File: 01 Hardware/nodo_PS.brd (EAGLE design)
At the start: 73 x 93 mm, 31 parts, among them IC1 ATMEGA3208-XU, SW1 EG1213

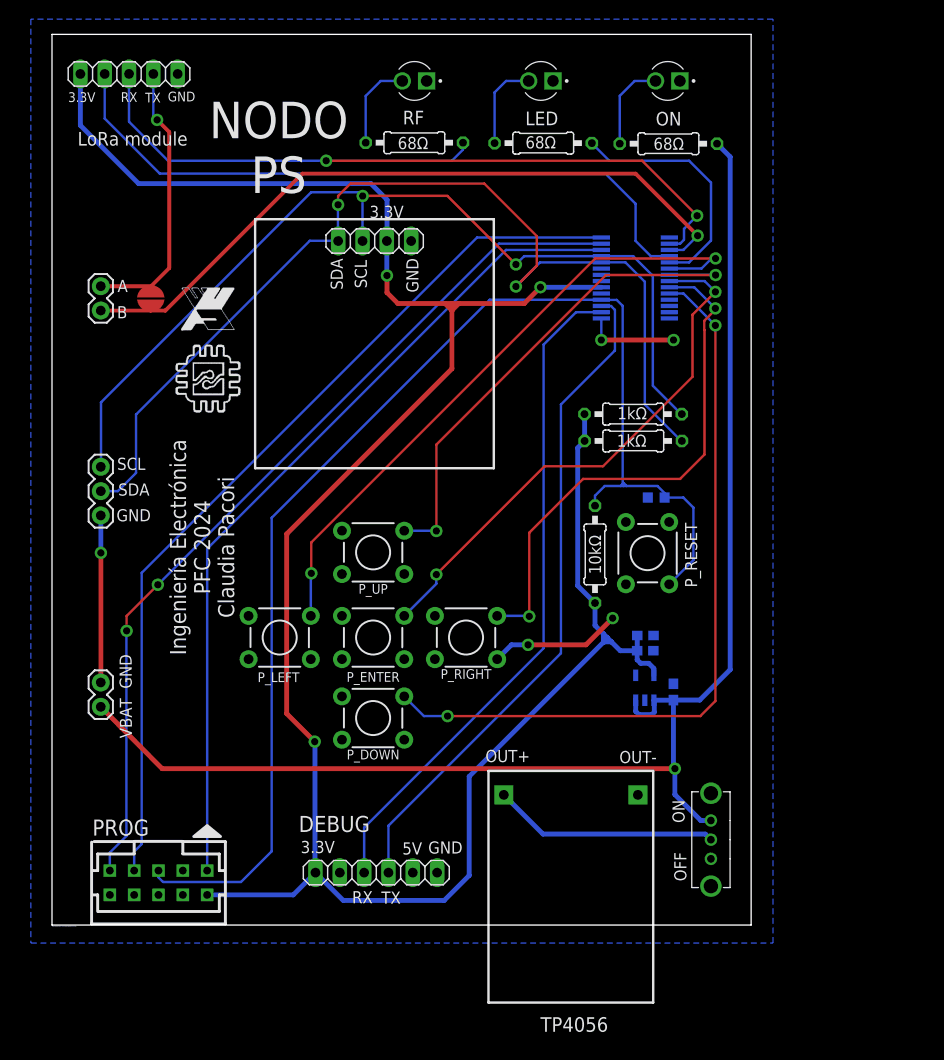
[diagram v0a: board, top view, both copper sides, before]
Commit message: actualizacion de archivos 24-2
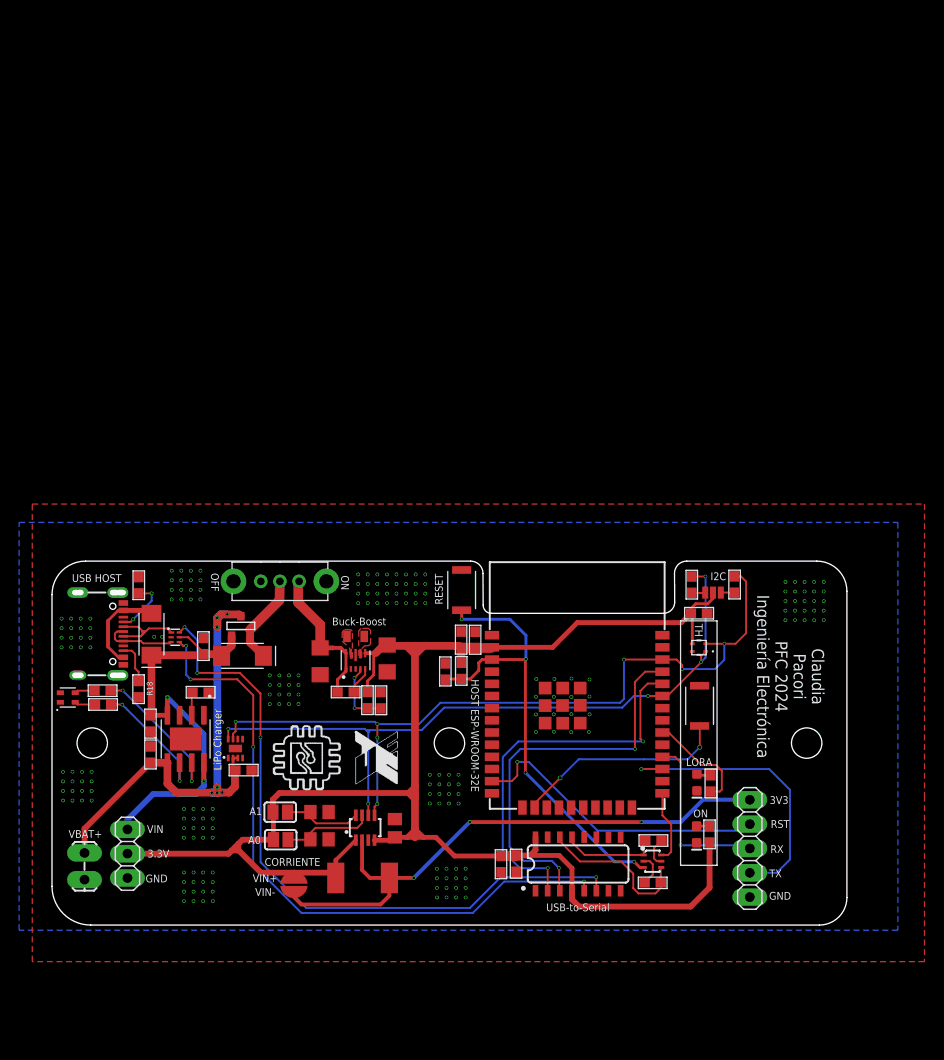
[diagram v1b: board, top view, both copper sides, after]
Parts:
- removed BAT: TP4056MODULE, TP4056MODULE:TP4056MODULE
- removed C4: 1.0uF, SparkFun-Capacitors:0603@3
- removed C5: 0.1uF, SparkFun-Capacitors:0603
- removed DEBUG: (no value), pinhead:1X06
- removed IC1: ATMEGA3208-XU, ATMEGA3208-XU:SOP65P780X200-28N
- removed LORA: REYAX, pinhead:1X05
- removed L_ON1, L_ON2, L_ON3: LED_3MM, LED_3MM:LEDRD254W50D405H1055
- removed OLED: (no value), pinhead:1X04
- removed P_DOWN, P_ENTER, P_LEFT, P_RESET, P_RIGHT, P_UP: MOMENTARY-SWITCH-SPST-PTH-6.0MM, SparkFun-Switches:TACTILE_SWITCH_PTH_6.0MM
- removed R8: 10k, rcl:0207/10
- removed REG: 3.3V, SparkFun-IC-Power:SOT23-5
- removed SV1: (no value), con-harting-ml:3M_10
- removed TP1: (no value), SparkFun-Connectors:1X03
- removed TP3, TP4: (no value), SparkFun-Connectors:1X02
- added A0, A1: (no value), microbuilder:SOLDERJUMPER_REFLOW_NOPASTE
- added C11, C17, C3, C8: 0.1uF, SparkFun-Capacitors:0603
- added C14: 10uF, SparkFun-Capacitors:1206
- added C15: 22uF, SparkFun-Capacitors:1206
- added C16, C18: 4.7uF, SparkFun-Capacitors:0603
- added C2, C7: 10uF, SparkFun-Capacitors:0603
- added D1, D2: BLUE, SparkFun-LED:LED-0603
- added D3, D7: SS34, SparkFun-DiscreteSemi:DO-214AC
- added D5: PRTR5V0U2F, SparkFun-IC-Power:SOT886
- added D8: TJ-S1615SW6TGLCCSRGB-A5, SMD_RGB_:LED_OSTB0603C1C
- added J1: (no value), SparkFun-Connectors:1X02_LOCK_LONGPADS
- added J2: USB Female Type C Connector, SparkFun-Connectors:USB-C-16P_4LAYER-PADS
- added J3: REYAX, pinhead:1X05
- added JP2: (no value), pinhead:1X03
- added L1: 470nH, SparkFun-Coils:0805
- added R10, R12, R22, R23: 220, SparkFun-Resistors:0603
- added R11, R9: 10k, rcl:R0805
- added R13: 511k, SparkFun-Resistors:0603
- added R14: 91k, SparkFun-Resistors:0603
- added R15: 100k, SparkFun-Resistors:0603
- added R18, R19: 5.1k, SparkFun-Resistors:0603
- added R21: 1.2k, SparkFun-Resistors:0603
- added R3, R5: 10k, SparkFun-Resistors:0603
- added S1: EG1213, EG1213:SW_EG1213
- added SENSORCORRIENTE: INA219BIDCNT, microbuilder:SOT23-8
- added SW2: SKRKAEE020, SKRKAEE020:SKRKAEE020
- added T1: AO3401A, zetex:SOT-23
- added TH: SHT40-AD1B-R3, SHT40-AD1B-R3:SHT40AD1BR3
- added TP2: JUMPER-SMT_3_NO_NO-SILK, SparkFun-Jumpers:SMT-JUMPER_3_NO_NO-SILK
- added U11: TPS63802DLAR, TPS63802DLAR:VREG_TPS63802DLAR
- added U13: TP4056, TP4056:SOP127P600X175-9N
- added U2: ESP-WROOM-32E, SparkFun-RF:ESP-WROOM-32D-NARROW
- added U4: CH340C, SparkFun-IC-Comms:SO016
- added U5: MBT3904DW1T1, SparkFun-DiscreteSemi:SC70-6
- added U7: MAX17048, SparkFun-IC-Power:DFN-8
- C1: device rcl:C0603K -> SparkFun-Capacitors:0603
- C6: value 1.0uF -> 0.1uF; device SparkFun-Capacitors:0603@3 -> rcl:C0805
- R1: value 68 -> 0.1/1% (PT2512FK-070R1L); device rcl:0207/10 -> microbuilder:2512
- R2, R4: value 68 -> 10k; device rcl:0207/10 -> SparkFun-Resistors:0603
- R6: value 1k -> 10k; device rcl:0207/10 -> SparkFun-Resistors:0603
- R7: value 1k -> 150k; device rcl:0207/10 -> SparkFun-Resistors:0603
- SW1: value EG1213 -> SKRKAEE020; device EG1213:SW_EG1213 -> SKRKAEE020:SKRKAEE020
- moved R1 83.0 mm to (32.4, 4.92)
- moved JP1 63.0 mm to (25.3, 4.20), turned to 270 degrees
- moved R2 55.8 mm to (42.7, 26.5), turned to 90 degrees
- moved R4 54.5 mm to (66.8, 35.5), turned to 270 degrees
- moved R7 51.0 mm to (15.8, 29.1), turned to 270 degrees
- moved R6 41.8 mm to (62.8, 8.83), turned to 0 degrees
- moved SW1 36.8 mm to (42.8, 35.0), turned to 270 degrees
- moved C6 32.4 mm to (35.8, 10.1), flipped to the top
- moved C1 24.0 mm to (44.2, 29.8), flipped to the top, turned to 90 degrees
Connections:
- removed net DEBUG_RX: DEBUG.3, IC1.16
- removed net DEBUG_TX: DEBUG.4, IC1.17
- removed net LED: IC1.5, R2.1
- removed net LORA_RST: IC1.4, LORA.2
- removed net LORA_RX: IC1.2, LORA.3, R4.1
- removed net LORA_TXA: JP1.2, LORA.4, TP3.1
- removed net LORA_TXB: IC1.3, JP1.1, TP3.2
- removed net MISO: IC1.27, SV1.9
- removed net MOSI: IC1.26, SV1.1
- removed net N$2: L_ON2.A, R1.2
- removed net PULSE_ENTER: IC1.8, P_ENTER.3
- removed net PULSE_LEFT: IC1.6, P_LEFT.3
- removed net PULSE_RIGHT: IC1.9, P_RIGHT.3
- removed net PULS_DOWN: IC1.10, P_DOWN.3
- removed net PULS_UP: IC1.7, P_UP.3
- removed net RESET: C1.1, IC1.18, P_RESET.3, R8.1, SV1.5
- removed net SCK: IC1.28, SV1.7
- removed net SCL: IC1.25, OLED.2, R7.1, TP1.3
- removed net SDA: IC1.24, OLED.1, R6.1, TP1.2
- removed net SS: IC1.1
- removed net V_BATT: C6.1, R1.1, REG.1, REG.3, SW1.3, TP4.2
- new net ADDR0: A0.2, R9.2, SENSORCORRIENTE.7
- new net ADDR1: A1.2, R11.2, SENSORCORRIENTE.8
- new net CC1: J2.B5, R18.2
- new net CC2: J2.A5, R19.2
- new net CH_!CHRG: D8.3, R23.1
- new net CH_!STDBY: D8.2, R22.1
- new net CURRENT_MSR: J3.1, JP1.2, R1.1, SENSORCORRIENTE.2
- new net ESP16_RX2/LORA_TX: J3.4, U2.27
- new net ESP17_TX2/LORA_RX: J3.3, U2.28
- new net ESP1_TX1/USB_RX: U2.35, U4.3
- new net ESP32_!DTR: R6.1, U4.13, U5.1
- new net ESP32_!RTS: R5.1, U4.14, U5.4
- new net ESP32_EN: C3.1, R2.1, SW1.2, U2.3, U5.3
- new net ESP3_RX1/USB_TX: U2.34, U4.2
- new net ESP_0/BOOT: U2.25, U5.6
- new net ESP_13/AUX: SW2.2, U2.16
- new net ESP_14/LORA_RST: J3.2, U2.13
- new net ESP_18/LORA_ST: R12.2, U2.30
- new net ESP_21/SDA: R4.1, SENSORCORRIENTE.6, TH.1, U2.33, U7.8
- new net ESP_22/SCL: R3.1, SENSORCORRIENTE.5, TH.2, U2.36, U7.7
- new net N$10: L1.2, U11.7
- new net N$11: R22.2, U13.6
- new net N$12: R13.1, R14.2, U11.4
- new net N$13: R23.2, U13.7
- new net N$14: R3.2, TP2.3
- new net N$15: R4.2, TP2.1
- new net N$18: R15.1, U11.5
- new net N$24: R6.2, U5.5
- new net N$25: R5.2, U5.2
- new net N$31: R21.2, U13.2
- new net N$4: D5.6, U4.6
- new net N$5: D1.A, R10.1
- new net N$7: D2.A, R12.1
- new net N$8: L1.1, U11.9
- new net USB-C-D+: D5.3, J2.A6, J2.B6
- new net VBAT: C17.1, C18.1, J1.2, T1.1, U13.5, U7.2, U7.3
- new net VBUS: D7.A, J2.VBUS1, J2.VBUS2
- new net VCC: D3.C, S1.2, T1.2
- new net VIN_S: C14.1, R15.2, S1.1, U11.1, U11.10
- net 3.3V: now also A0.1, A1.1, C1.1, C11.1, C15.1, C2.1, C6.1, C7.1, C8.1, JP1.1, JP2.2, R1.2, R10.2, R13.2, R2.2, SENSORCORRIENTE.1, SENSORCORRIENTE.4, TH.3, TP2.2, U11.6, U2.2, U4.16, U4.4; no longer C4.1, C5.2, DEBUG.1, IC1.20, LORA.1, OLED.3, R6.2, R7.2, R8.2, REG.5, SV1.2
- net GND: now also C11.2, C14.2, C15.2, C16.2, C17.2, C18.2, C2.2, C3.2, C7.2, C8.2, D1.C, D2.C, D5.2, D8.4, J1.1, J2.GND, J2.GND2, J2.SHLD2, J2.SHLD3, J2.SHLD4, J2.SHLD5, J3.5, JP2.3, R11.1, R14.1, R18.1, R19.1, R21.1, R7.1, R9.1, SENSORCORRIENTE.3, SW2.1, TH.4, U11.2, U11.3, U11.8, U13.1, U13.3, U13.9, U2.1, U2.15, U2.38, U2.GND1, U2.GNDT1, U2.GNDT2, U2.GNDT3, U2.GNDT4, U2.GNDT5, U2.GNDT6, U2.GNDT7, U2.GNDT8, U4.1, U7.1, U7.4, U7.6, U7.9; no longer BAT.6, C4.2, C5.1, DEBUG.6, IC1.15, IC1.21, LORA.5, L_ON1.C, L_ON2.C, L_ON3.C, OLED.4, P_DOWN.1, P_ENTER.1, P_LEFT.1, P_RESET.1, P_RIGHT.1, P_UP.1, REG.2, SV1.10, SV1.3, SV1.4, SV1.6, SV1.8, TP1.1, TP4.1
- net N$1: now also D5.1, J2.A7, J2.B7; no longer L_ON3.A, R2.2
- net N$3: now also D5.4, U4.5; no longer L_ON1.A, R4.2
- net VIN: now also C16.1, D3.A, D5.5, D7.C, JP2.1, R7.2, T1.3, U13.4, U13.8; no longer BAT.3, SW1.2
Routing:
- net V_BATT: track 146.8 -> 0.00 mm, vias 1 -> 0
- net RESET: track 137.0 -> 0.00 mm
- net SDA: track 107.2 -> 0.00 mm, vias 2 -> 0
- net SCL: track 98.2 -> 0.00 mm, vias 2 -> 0
- net SCK: track 93.9 -> 0.00 mm
- net MISO: track 93.0 -> 0.00 mm, vias 2 -> 0
- net LORA_RX: track 88.6 -> 0.00 mm, vias 2 -> 0
- net MOSI: track 87.7 -> 0.00 mm
- net ESP_22/SCL: track 0.00 -> 82.1 mm, vias 0 -> 7
- net PULS_DOWN: track 79.4 -> 0.00 mm, vias 2 -> 0
- net ESP_21/SDA: track 0.00 -> 74.8 mm, vias 0 -> 5
- net LORA_TXB: track 74.5 -> 0.00 mm, vias 1 -> 0
- net LORA_RST: track 71.8 -> 0.00 mm
- net N$4: track 0.00 -> 71.0 mm, vias 0 -> 4
- net DEBUG_RX: track 70.3 -> 0.00 mm
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- added copper zone on layer 1, net GND
- added copper zone on layer 1, net N$10
- added copper zone on layer 1, net N$8
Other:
- board size 73 x 93 mm -> 83 x 38 mm
- board text added: "3V3"
- board text added: "Buck-Boost"
- board text added: "CORRIENTE"
- board text added: "Claudia Pacori PFC 2024 Ingeniería Electrónica"
- board text added: "HOST ESP-WROOM-32E"
- board text added: "I2C"
- board text added: "LORA"
- board text added: "LiPo Charger"
- board text added: "RESET"
- board text added: "RST"
- board text added: "TH"
- board text added: "USB HOST"
- board text added: "USB-to-Serial"
- board text added: "VBAT+"
- board text added: "VIN"
- board text added: "VIN+"
- board text added: "VIN-"
- board text removed: "0.1uF"
- board text removed: "10kΩ"
- board text removed: "1kΩ"
- board text removed: "1uF"
- board text removed: "5V"
- board text removed: "68Ω"
- board text removed: "A"
- board text removed: "ATMEGA"
- board text removed: "B"
- board text removed: "C:/Users/Claudia/Documents/03 Tesis/01 Hardware/imagenes/ELECTRONICA2.bmp"
- board text removed: "C:/Users/Claudia/Documents/03 Tesis/01 Hardware/imagenes/LOGO_UTEC2.bmp"
- board text removed: "DEBUG"
- board text removed: "Ingeniería Electrónica PFC 2024 Claudia Pacori"
- board text removed: "LED"
- board text removed: "LoRa module"
- board text removed: "NODO PS"
- board text removed: "OUT+"
- board text removed: "OUT-"
- board text removed: "PROG"
- board text removed: "RF"
- board text removed: "SCL"
- board text removed: "SDA"
- board text removed: "VBAT"
